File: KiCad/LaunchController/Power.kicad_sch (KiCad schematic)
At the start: 38 parts, among them J1 DC_IN, J8 CONN_CONVERTER, Q1 TJ8S06M3L, Q2 2SC3325-Y, Q3 TJ8S06M3L, U3 INA219BIDCNT, U5 INA219BIDCNT

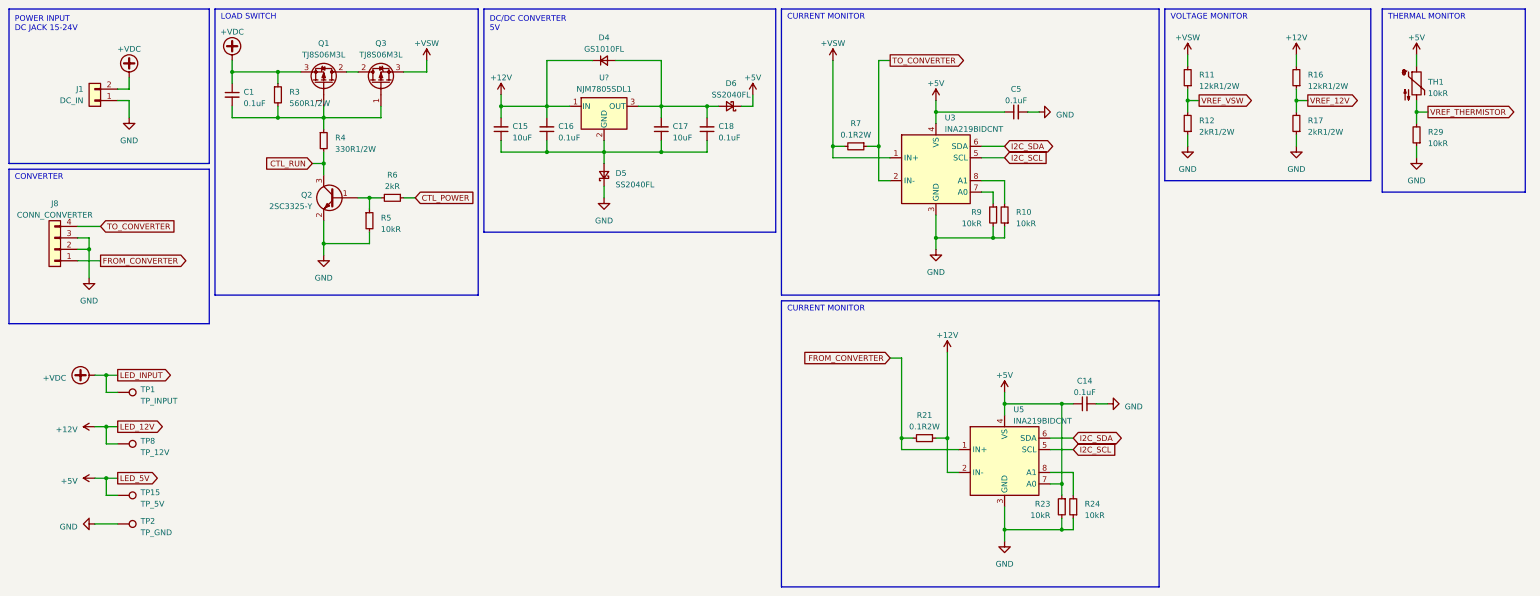
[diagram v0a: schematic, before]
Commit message: さらに分割
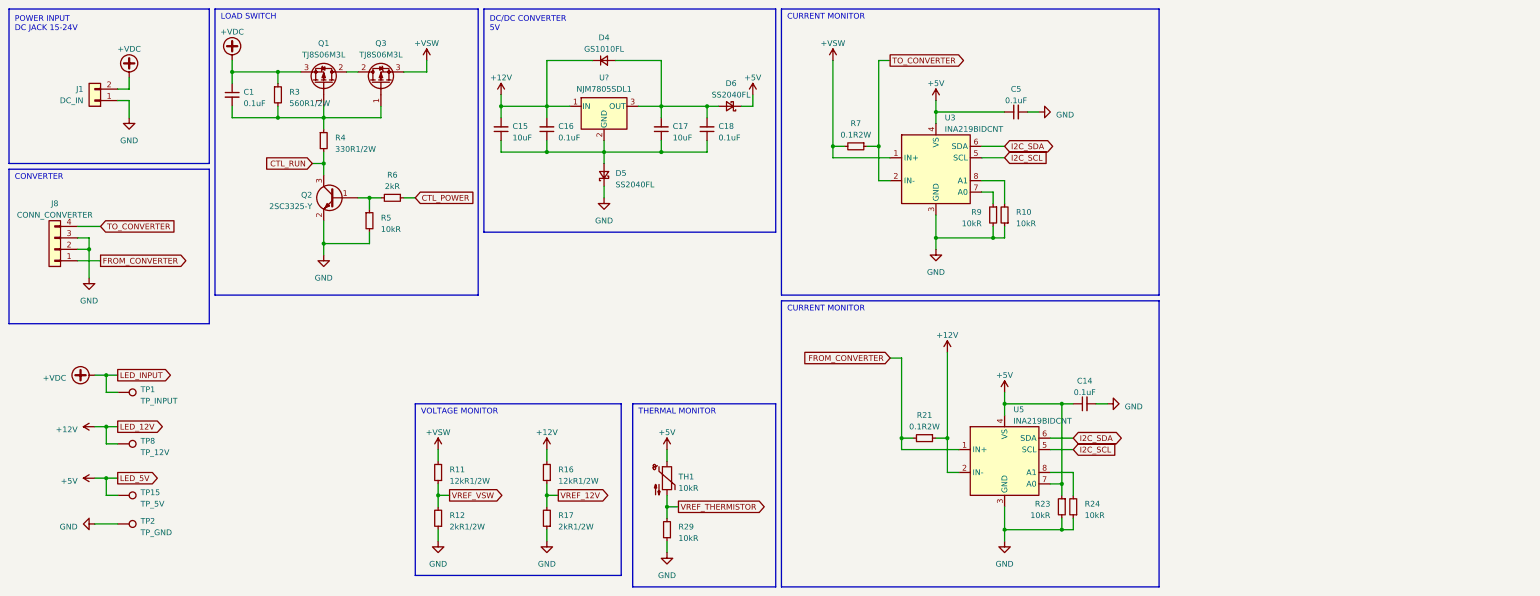
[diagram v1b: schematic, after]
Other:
- moved on the sheet: R11, R12, R16, R17, R29, TH1
